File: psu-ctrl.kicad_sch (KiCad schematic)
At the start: 31 parts, among them J4 Conn_02x20_Odd_Even, U5 12A

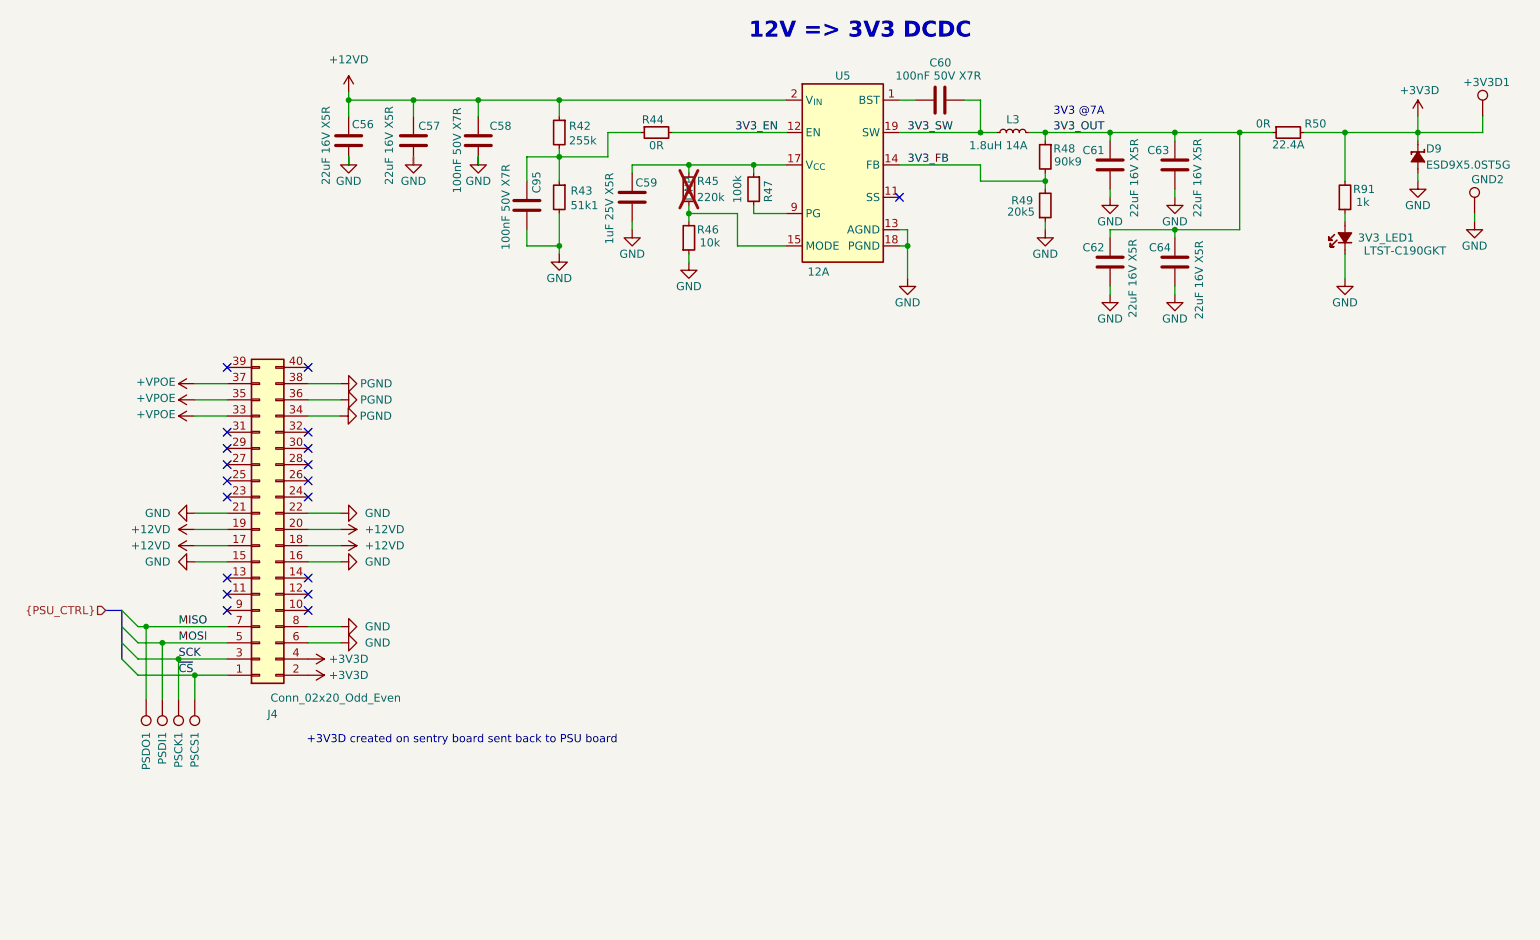
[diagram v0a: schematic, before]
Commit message: latestL
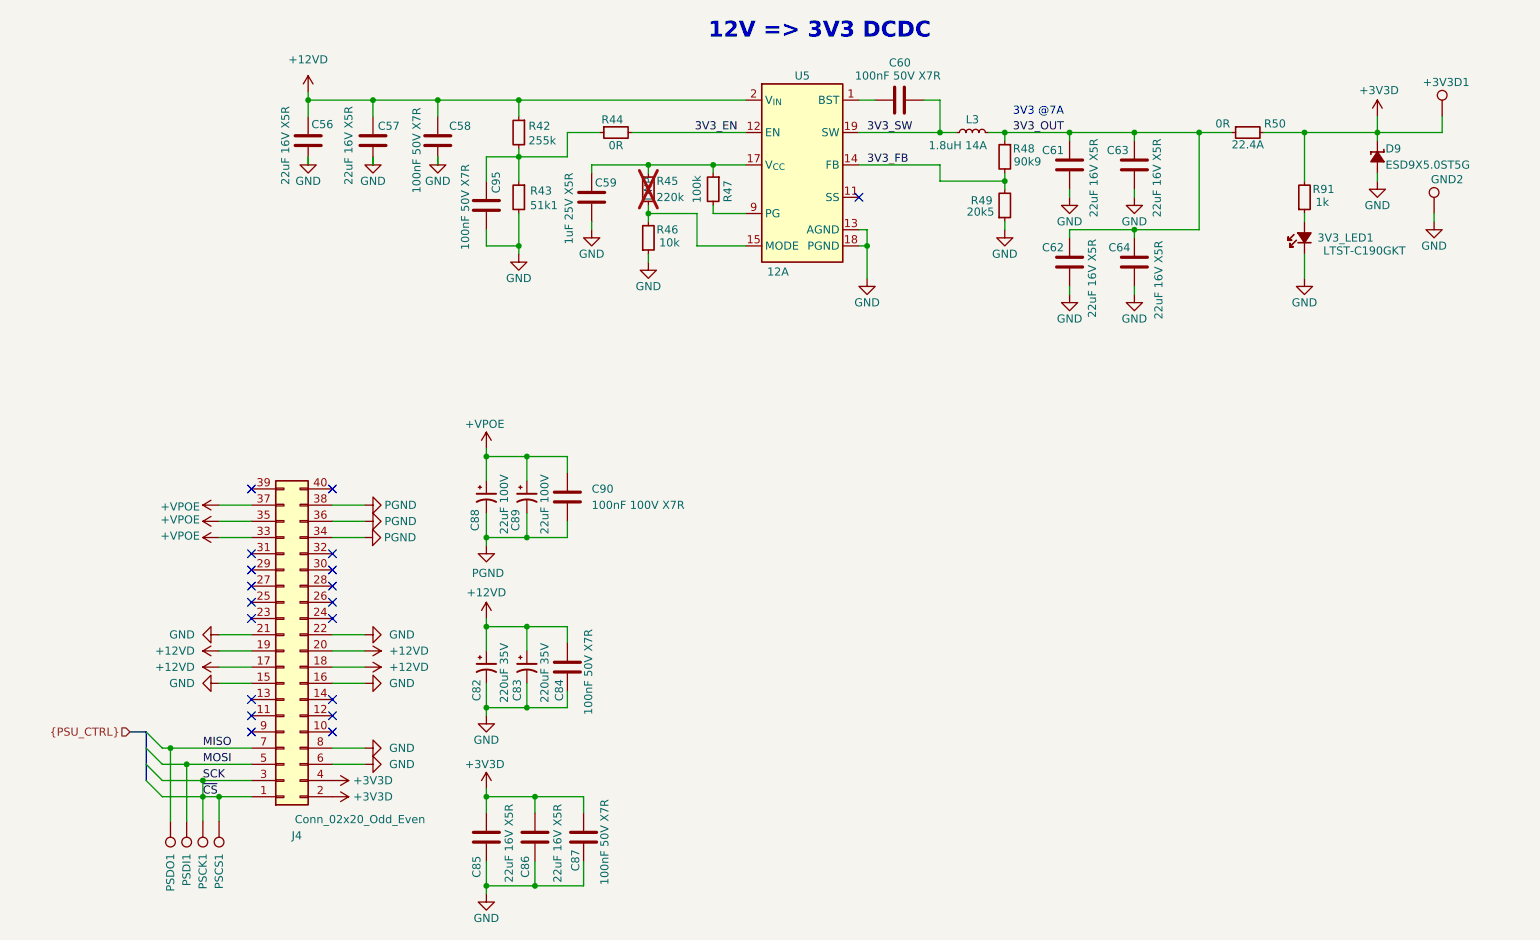
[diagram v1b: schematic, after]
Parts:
- added C82, C83: 220uF 35V, Capacitor_SMD:CP_Elec_8x10.5, symbol andium-capacitors:ALUM_SMT_220uF_35V_W8_H10.2MM_EMZA350ARA221MHA0G
- added C84, C87: 100nF 50V X7R, andium-capacitors:C_0402_1005Metric, symbol andium-capacitors:CER_100nF_50V_X7R_0402
- added C85, C86: 22uF 16V X5R, antmicro-footprints:C_0603_1608Metric, symbol andium-capacitors:CER_22uF_16V_X5R_0603
- added C88, C89: 22uF 100V, Capacitor_SMD:CP_Elec_8x10.5, symbol andium-capacitors:ALUM_SMT_22uF_100V_W8_H10.5MM_UUX2A220MNL6GS
- added C90: 100nF 100V X7R, andium-capacitors:C_0603_1608Metric, symbol andium-capacitors:CER_100nF_100V_X7R_0603
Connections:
- net +12VD: now also C82.1, C83.1, C84.1
- net +3V3D: now also C85.1, C86.1, C87.1
- net +VPOE: now also C88.1, C89.1, C90.1
- net GND: now also C82.2, C83.2, C84.2, C85.2, C86.2, C87.2
- net PGND: now also C88.2, C89.2, C90.2
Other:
- note removed: "+3V3D created on sentry board sent back to PSU board"
- moved on the sheet: +3V3D1, 3V3_LED1, C56, C57, C58, C59, C60, C61, C62, C63, C64, C95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
